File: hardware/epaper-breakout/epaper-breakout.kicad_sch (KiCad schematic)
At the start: 107 parts, among them J1 XF2M-3315-1A, J2 C10418, J3 Conn_02x05_Counter_Clockwise, J4 ED060SC4, J5 Conn_01x02_Female, J7 Conn_01x12, Q3 MMBT3904, Q4 MMBT3904, U1 MCP1700-3302E_SOT23, U11 TP4056, U12 CH340C, U2 PCA9535PW, U3 TPS651851RSLR, U4 XC6206PxxxMR, U6 ED060XC5, U7 TPS2113APW

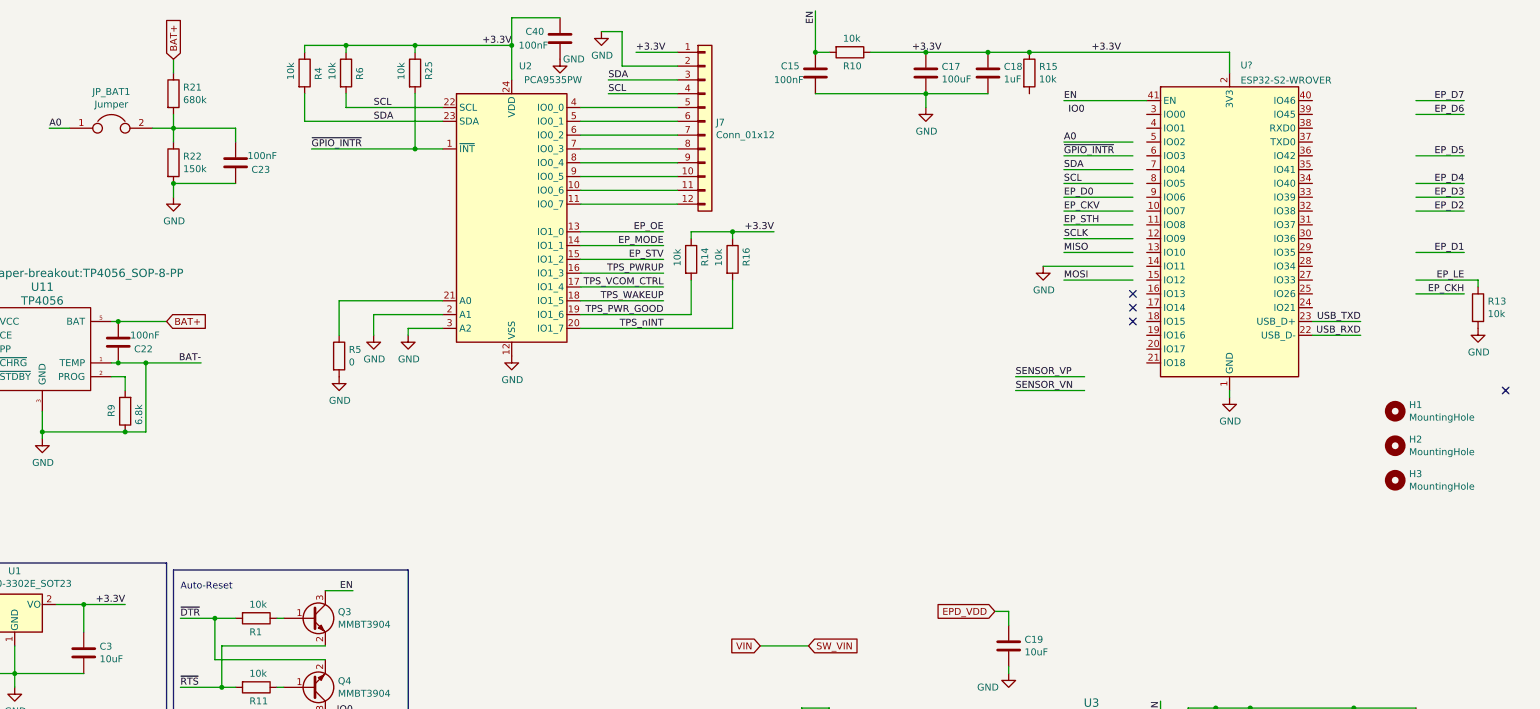
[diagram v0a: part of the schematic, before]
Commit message: #1 sch
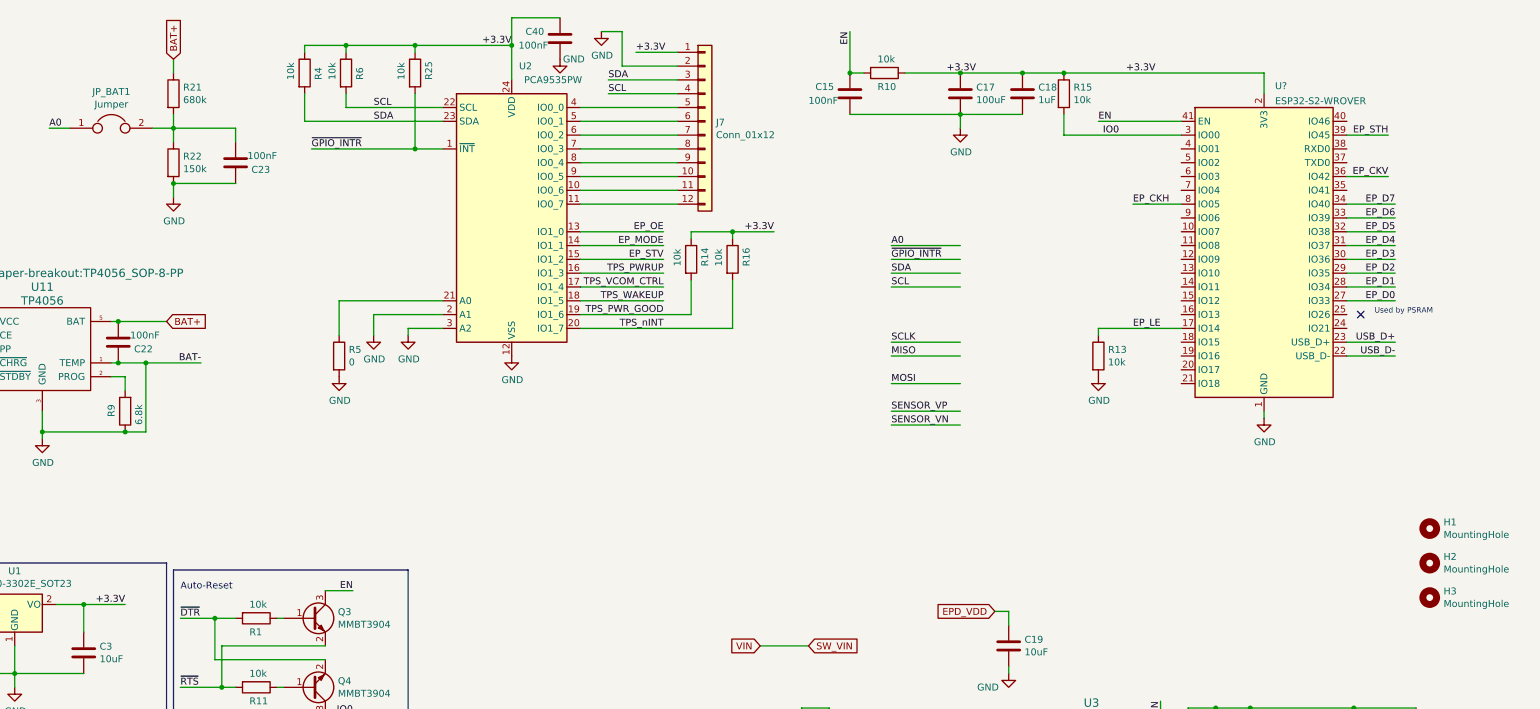
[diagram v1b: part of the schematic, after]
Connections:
- net EP_CKH: now also U?.8 (IO05)
- net EP_CKV: now also U?.36 (IO42)
- net EP_D0: now also U?.27 (IO33)
- net EP_D1: now also U?.28 (IO34)
- net EP_D2: now also U?.29 (IO35)
- net EP_D3: now also U?.30 (IO36)
- net EP_D4: now also U?.31 (IO37)
- net EP_D5: now also U?.32 (IO38)
- net EP_D6: now also U?.33 (IO39)
- net EP_D7: now also U?.34 (IO40)
- net EP_LE: now also U?.17 (IO14)
- net EP_STH: now also U?.39 (IO45)
- net IO0: now also R15.2, U?.3 (IO00)
- net USB_D+: now also U?.23 (USB_D+)
- net USB_D-: now also U?.22 (USB_D-)
- net USB_RXD: no longer U?.22 (USB_D-)
- net USB_TXD: no longer U?.23 (USB_D+)
- no-connect marks 26 -> 23
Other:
- note added: "Used by PSRAM"
- moved on the sheet: C15, C17, C18, H1, H2, H3, R10, R13, R15, U?
